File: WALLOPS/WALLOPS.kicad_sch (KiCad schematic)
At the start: 20 parts, among them J1 JST-PH 1x8 Connector - WALLOP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, Q1 AO3401A, U1 VL53L8CX 0 (Zwicky), U2 VL58L8CX 1 (Aristotle), U3 VL53L8CX 3 (Copernicus), U4 VL53L8CX 2 (Brahe), U5 6DOF IMU (Sisko), U6 5V to 3.3V Converter

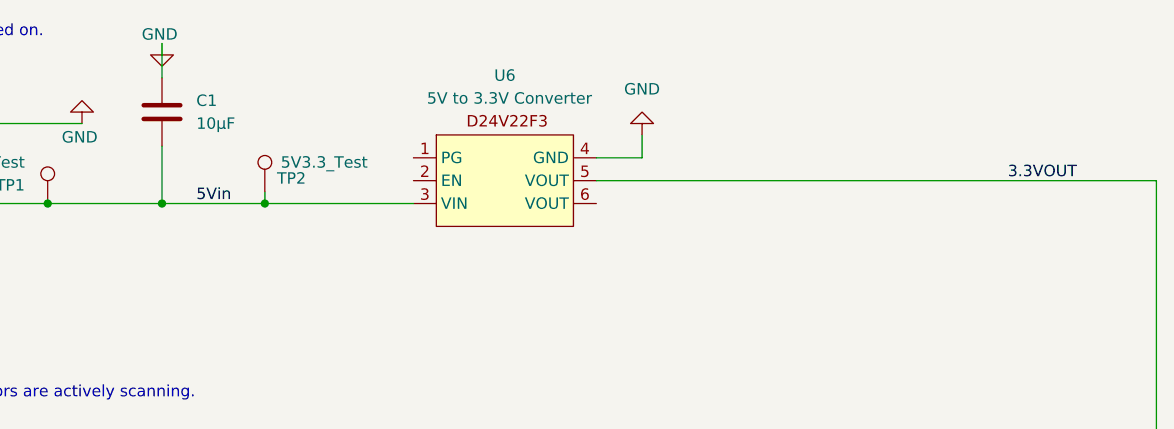
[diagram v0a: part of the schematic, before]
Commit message: Added updated WALLOPS PCB
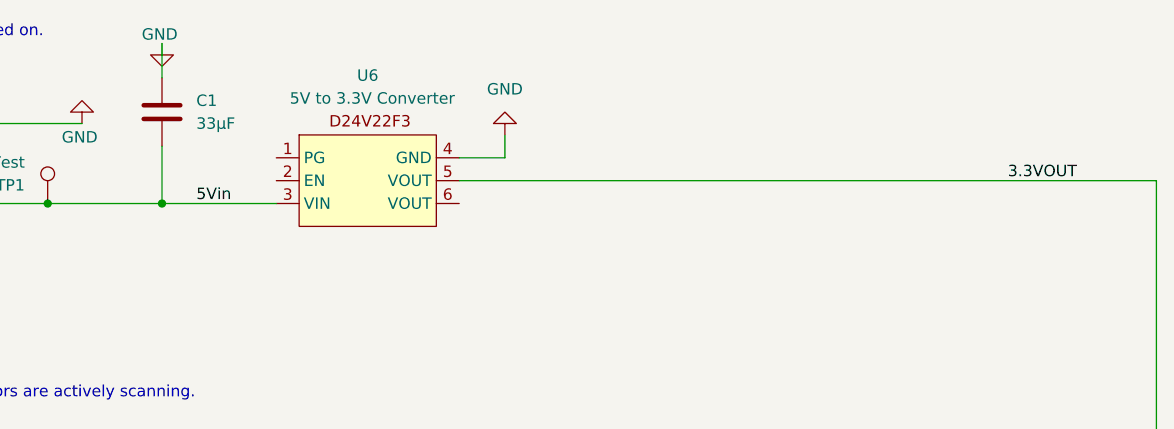
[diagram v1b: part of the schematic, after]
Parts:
- removed TP2: 5V3.3_Test, RockSat:TestPoint_Pad_D2.0mm_With_Tolerance, symbol Connector:TestPoint
- C1: value 10µF -> 33µF
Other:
- moved on the sheet: U6
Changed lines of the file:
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@@
 	)
 	(junction
-		(at 148.59 43.18)
-		(diameter 0)
-		(color 0 0 0 0)
-	)
-	(junction
 		(at 90.17 81.28)
 		(diameter 0)
@@
 	(wire
 		(pts
-			(xy 185.42 40.64) (xy 247.65 40.64)
+			(xy 170.18 40.64) (xy 247.65 40.64)
 		)
 		(stroke
@@
 	(wire
 		(pts
-			(xy 137.16 43.18) (xy 148.59 43.18)
-		)
-		(stroke
-			(width 0)
-			(type default)
-		)
-	)
-	(wire
-		(pts
 			(xy 128.27 144.78) (xy 128.27 151.13)
 		)
@@
 	(wire
 		(pts
-			(xy 190.5 35.56) (xy 190.5 38.1)
+			(xy 175.26 35.56) (xy 175.26 38.1)
 		)
 		(stroke
@@
 	(wire
 		(pts
-			(xy 185.42 38.1) (xy 190.5 38.1)
+			(xy 170.18 38.1) (xy 175.26 38.1)
 		)
 		(stroke
@@
 	(wire
 		(pts
-			(xy 148.59 43.18) (xy 165.1 43.18)
+			(xy 137.16 43.18) (xy 149.86 43.18)
 		)
 		(stroke
@@
 	(wire
 		(pts
-			(xy 148.59 41.91) (xy 148.59 43.18)
-		)
-		(stroke
-			(width 0)
-			(type default)
-		)
-	)
-	(wire
-		(pts
 			(xy 64.77 68.58) (xy 64.77 81.28)
 		)
@@
 			)
 		)
-		(property "Value" "10µF"
+		(property "Value" "33µF"
 			(at 140.97 34.2899 0)
 			(effects
@@
 	(symbol
 		(lib_id "Connector:TestPoint")
-		(at 148.59 41.91 0)
-		(unit 1)
-		(exclude_from_sim no)
-		(in_bom yes)
-		(on_board yes)
-		(dnp no)
-		(property "Reference" "TP2"
-			(at 153.162 40.386 0)
-			(effects
-				(font
-					(size 1.27 1.27)
-				)
-				(justify right)
-			)
-		)
-		(property "Value" "5V3.3_Test"
-			(at 160.02 38.608 0)
-			(effects
-				(font
-					(size 1.27 1.27)
-				)
-				(justify right)
-			)
-		)
-		(property "Footprint" "RockSat:TestPoint_Pad_D2.0mm_With_Tolerance"
-			(at 153.67 41.91 0)
-			(effects
-				(font
-					(size 1.27 1.27)
-				)
-				(hide yes)
-			)
-		)
-		(property "Datasheet" "~"
-			(at 153.67 41.91 0)
-			(effects
-				(font
-					(size 1.27 1.27)
-				)
-				(hide yes)
-			)
-		)
-		(property "Description" "test point"
-			(at 148.59 41.91 0)
-			(effects
-				(font
-					(size 1.27 1.27)
-				)
-				(hide yes)
-			)
-		)
-		(pin "1"
-		)
-		(instances
-			(project ""
-				(path "/a71b320d-cbec-40c8-adfb-8ac61cfef5bf"
-					(reference "TP2")
-					(unit 1)
-				)
-			)
-		)
-	)
-	(symbol
-		(lib_id "Connector:TestPoint")
 		(at 60.96 101.6 180)
 		(unit 1)
@@
 	(symbol
 		(lib_id "RockSat_Sym:Pololu_D24V22F3")
-		(at 175.26 40.64 0)
+		(at 160.02 40.64 0)
 		(unit 1)
 		(exclude_from_sim no)
@@
 		(dnp no)
 		(property "Reference" "U6"
-			(at 175.26 28.956 0)
+			(at 160.02 28.956 0)
 			(effects
 				(font
@@
 		)
 		(property "Value" "5V to 3.3V Converter"
-			(at 175.768 31.496 0)
+			(at 160.528 31.496 0)
 			(effects
 				(font
@@
 		)
 		(property "Footprint" "RockSat:D24V22F3"
-			(at 175.26 40.64 0)
+			(at 160.02 40.64 0)
 			(effects
 				(font
@@
 		)
 		(property "Datasheet" ""
-			(at 175.26 40.64 0)
+			(at 160.02 40.64 0)
 			(effects
 				(font
@@
 		)
 		(property "Description" ""
-			(at 175.26 40.64 0)
+			(at 160.02 40.64 0)
 			(effects
 				(font
@@
 	(symbol
 		(lib_id "power:GND")
-		(at 190.5 35.56 180)
+		(at 175.26 35.56 180)
 		(unit 1)
 		(exclude_from_sim no)
@@
 		(fields_autoplaced yes)
 		(property "Reference" "#PWR02"
-			(at 190.5 29.21 0)
+			(at 175.26 29.21 0)
 			(effects
 				(font
@@
 		)
 		(property "Value" "GND"
-			(at 190.5 30.48 0)
+			(at 175.26 30.48 0)
 			(effects
 				(font
@@
 		)
 		(property "Footprint" ""
-			(at 190.5 35.56 0)
+			(at 175.26 35.56 0)
 			(effects
 				(font
@@
 		)
 		(property "Datasheet" ""
-			(at 190.5 35.56 0)
+			(at 175.26 35.56 0)
 			(effects
 				(font
@@
 		)
 		(property "Description" "Power symbol creates a global label with name \"GND\" , ground"
-			(at 190.5 35.56 0)
+			(at 175.26 35.56 0)
 			(effects
 				(font
